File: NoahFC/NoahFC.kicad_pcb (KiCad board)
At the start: 2 copper layers, 40 x 45 mm, 25 parts, among them J1 CH1, J10 GND, J2 CH2, J3 MPU6050, J4 FTDI, J5 8.4V, J6 CH3, J7 PPM, J8 GPS, J9 CH4, U1 ATmega328-A, U3 AMS1117-5.0, Y1 16Mhz

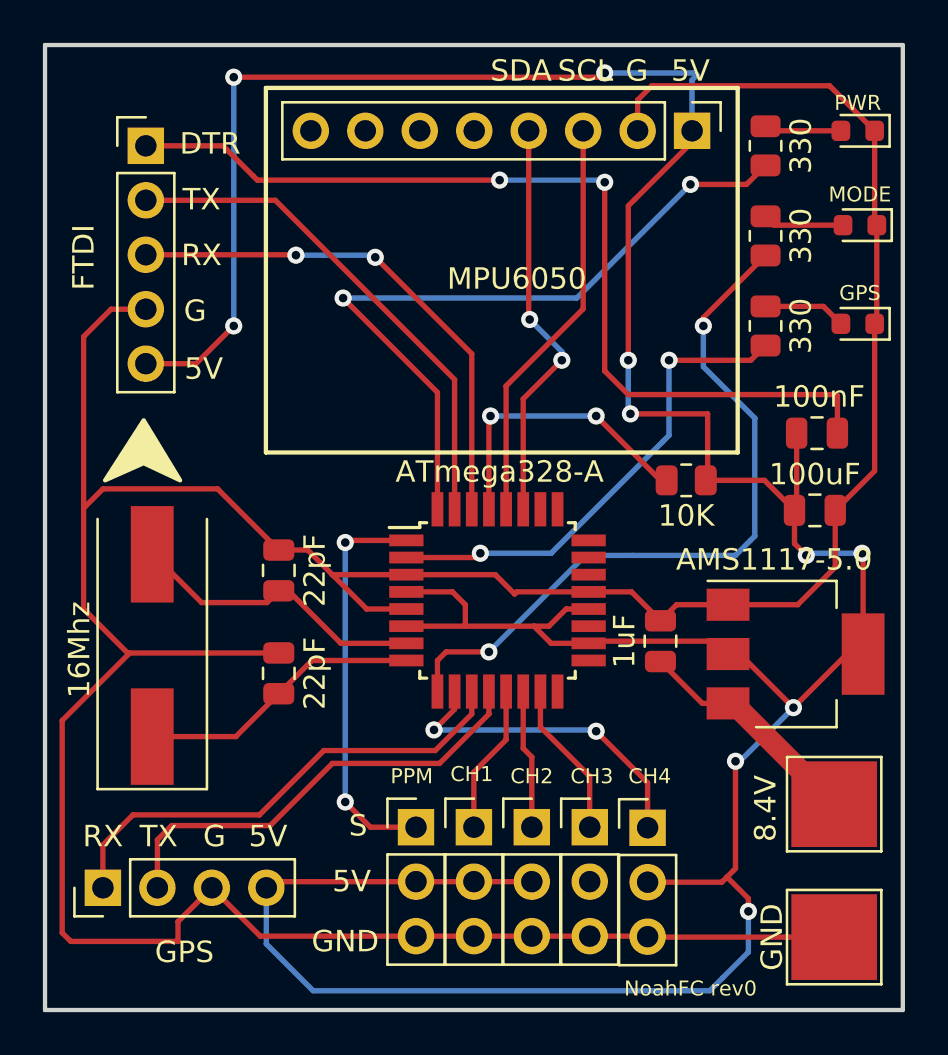
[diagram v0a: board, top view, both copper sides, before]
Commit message: revision 1
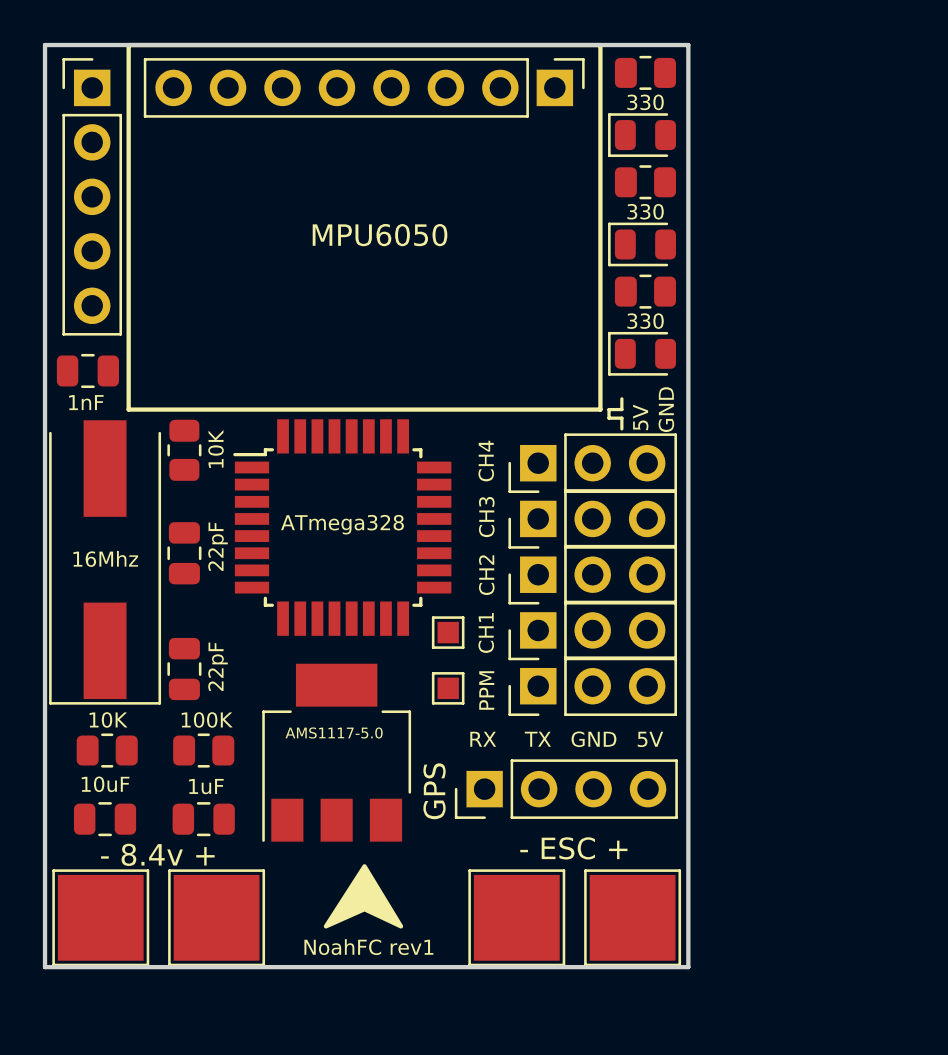
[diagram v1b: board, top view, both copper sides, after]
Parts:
- added J11: SCK, TestPoint:TestPoint_Pad_1.0x1.0mm, F.Cu at (150.8, 88.0)
- added J12: MISO, TestPoint:TestPoint_Pad_1.0x1.0mm, F.Cu at (150.8, 85.4)
- added J13: VCC, TestPoint:TestPoint_Pad_4.0x4.0mm, F.Cu at (159.4, 98.7)
- added J14: GND, TestPoint:TestPoint_Pad_4.0x4.0mm, F.Cu at (154.0, 98.7)
- added R5: 100K, Resistor_SMD:R_0805_2012Metric, F.Cu at (139.4, 90.9)
- added R6: 10K, Resistor_SMD:R_0805_2012Metric, F.Cu at (134.9, 90.9)
- C3: value 100nF -> 1nF
- C5: value 100uF -> 10uF
- D1, D2, D3: footprint LED_SMD:LED_0603_1608Metric -> LED_SMD:LED_0805_2012Metric
- J5: value 8.4V -> VCC
- U1: value ATmega328-A -> ATmega328
- moved C5 36.1 mm to (134.8, 94.1)
- moved J10 34.2 mm to (134.6, 98.7)
- moved C3 34.1 mm to (134.0, 73.2), turned to 180 degrees
- moved J5 29.3 mm to (140.0, 98.7)
- moved R1 23.4 mm to (138.5, 76.9), turned to -90 degrees
- moved C4 22.9 mm to (139.4, 94.1), turned to 0 degrees
- moved U3 21.9 mm to (145.6, 91.0), turned to 90 degrees
- moved J8 18.4 mm to (152.5, 92.7)
- moved J9 17.7 mm to (155.0, 77.5), turned to 90 degrees
- moved J6 14.6 mm to (155.0, 80.1), turned to 90 degrees
- moved D2 13.2 mm to (160.0, 62.2), turned to 0 degrees
- moved R3 13.1 mm to (160.0, 59.3), turned to 0 degrees
- moved J2 11.8 mm to (155.0, 82.7), turned to 90 degrees
- moved D3 11.7 mm to (160.0, 72.4), turned to 0 degrees
- moved D1 11.2 mm to (160.0, 67.3), turned to 0 degrees
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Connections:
- net Net-(C1-Pad1) renamed XTAL1
- net Net-(C2-Pad1) renamed XTAL2
- net Net-(U1-Pad2) renamed LED_MODE
- C3 pad 1: 5V -> RESET
- J1 pad 2: 5V -> 5V_BEC
- J2 pad 2: 5V -> 5V_BEC
- J6 pad 2: unconnected-(J6-Pad2) -> 5V_BEC
- J7 pad 2: 5V -> 5V_BEC
- J9 pad 2: 5V -> 5V_BEC
- R1 pad 1: Net-(R1-Pad1) -> RESET
- R2 pad 1: Net-(U1-Pad32) -> LED_GPS
- R4 pad 1: Net-(U1-Pad9) -> LED_PWR
- U1 pad 11: GPS_RX -> LED_PWR
- U1 pad 16: unconnected-(U1-Pad16) -> MISO
- U1 pad 17: unconnected-(U1-Pad17) -> SCK
- U1 pad 19: unconnected-(U1-Pad19) -> ADC6
- U1 pad 22: unconnected-(U1-Pad22) -> ADC7
- U1 pad 23: unconnected-(U1-Pad23) -> A0
- U1 pad 24: unconnected-(U1-Pad24) -> A1
- U1 pad 25: unconnected-(U1-Pad25) -> VOLTAGE_READ
- U1 pad 26: unconnected-(U1-Pad26) -> A3
- U1 pad 29: Net-(R1-Pad1) -> RESET
- U1 pad 32: Net-(U1-Pad32) -> GPS_RX
- U1 pad 9: Net-(U1-Pad9) -> LED_GPS
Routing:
- net 5V: track 166.3 -> 0.00 mm, vias 10 -> 0
- net GND: track 157.1 -> 0.00 mm
- net DTR: track 44.0 -> 0.00 mm, vias 2 -> 0
- net Net-(U1-Pad32): track 33.9 -> 0.00 mm, vias 2 -> 0
- net Net-(U1-Pad9): track 33.9 -> 0.00 mm, vias 2 -> 0
- net RX: track 24.4 -> 0.00 mm, vias 2 -> 0
- net TX: track 23.9 -> 0.00 mm
- net LED_MODE: track 22.9 -> 0.00 mm, vias 2 -> 0
- net GPS_RX: track 22.8 -> 0.00 mm
- net GPS_TX: track 21.2 -> 0.00 mm
- net SCL: track 19.1 -> 0.00 mm
- net SDA: track 19.0 -> 0.00 mm, vias 2 -> 0
- net PPM: track 18.8 -> 0.00 mm, vias 2 -> 0
- net CH4: track 15.3 -> 0.00 mm, vias 2 -> 0
- net XTAL1: track 14.0 -> 0.00 mm
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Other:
- board size 40 x 45 mm -> 30 x 43 mm
- board text added: "- 8.4v +"
- board text added: "- ESC +"
- board text added: "NoahFC rev1"
- board text added: "http://github.com/zosko/NoahFC by Bosko"
- board text removed: "G"
- board text removed: "NoahFC rev0"
- board text removed: "S"
